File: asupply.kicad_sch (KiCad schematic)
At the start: 73 parts

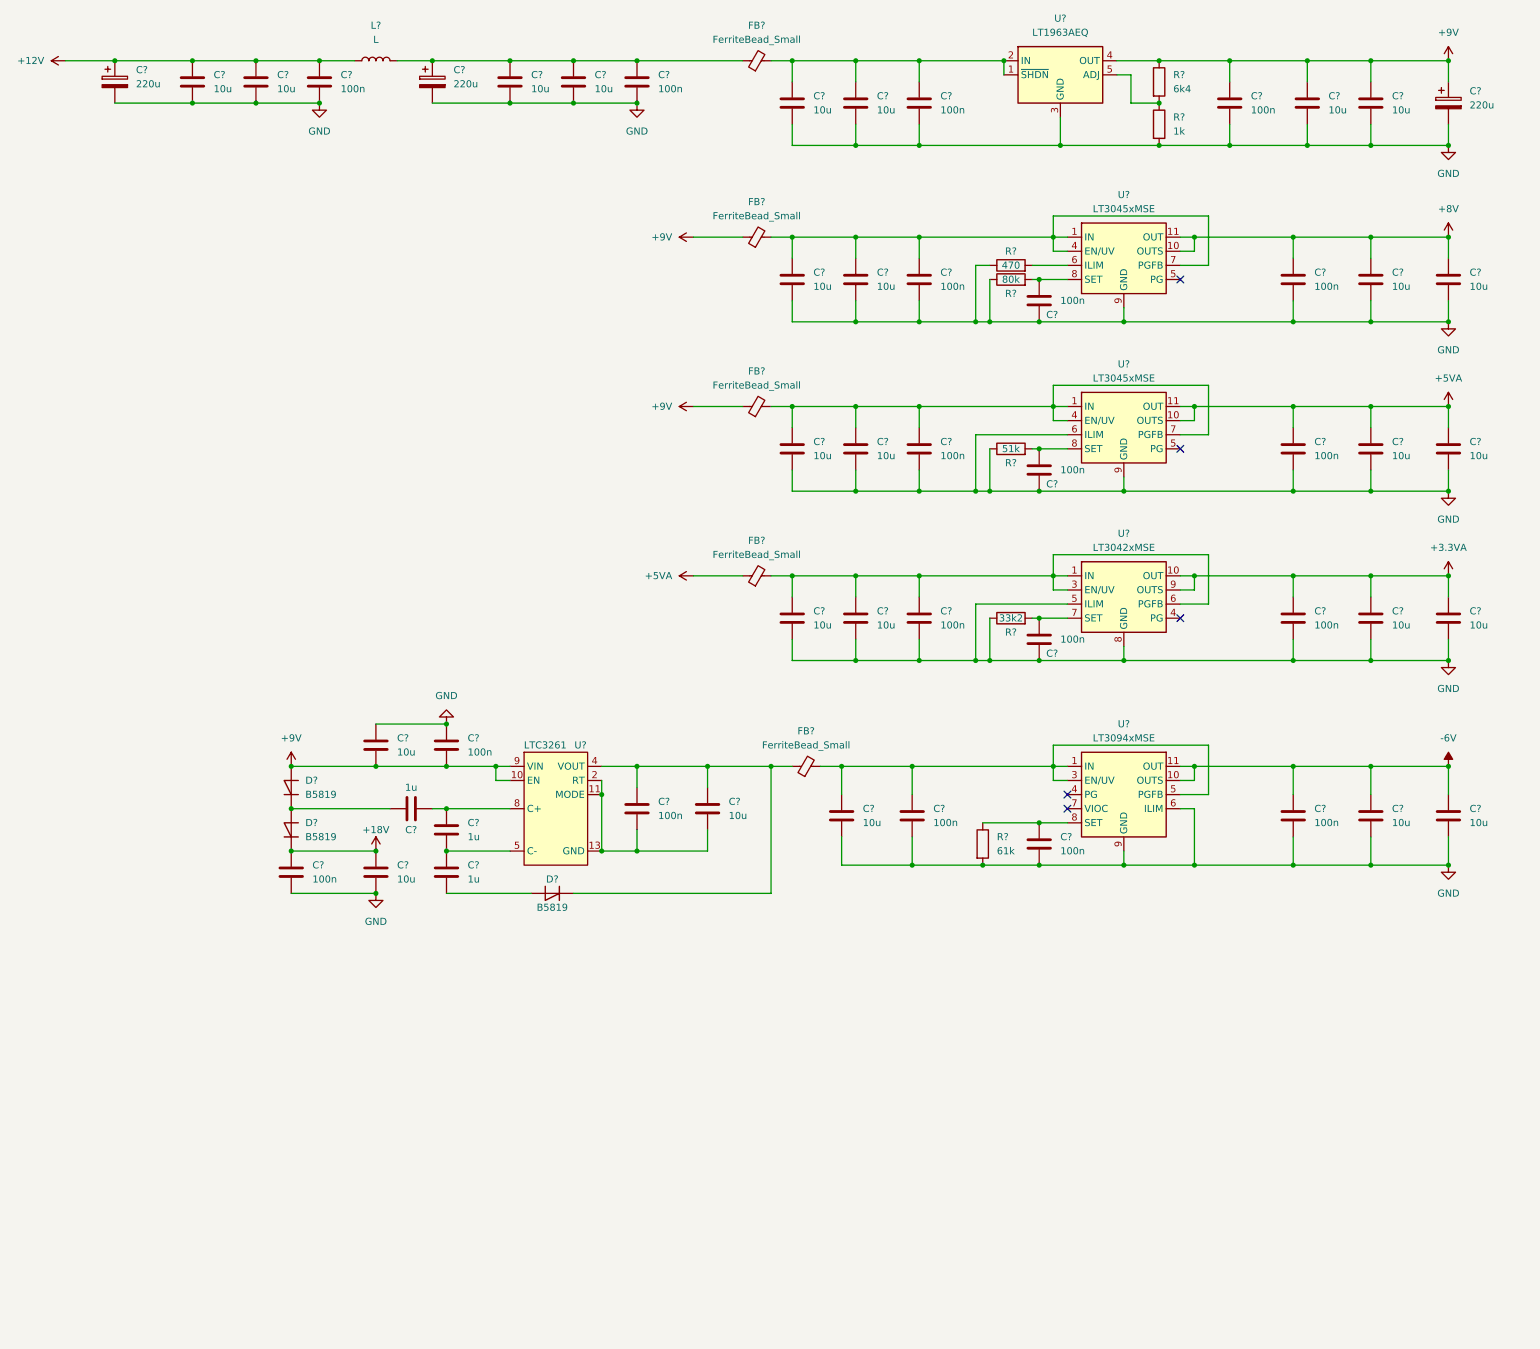
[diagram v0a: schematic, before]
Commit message: analog supply complete
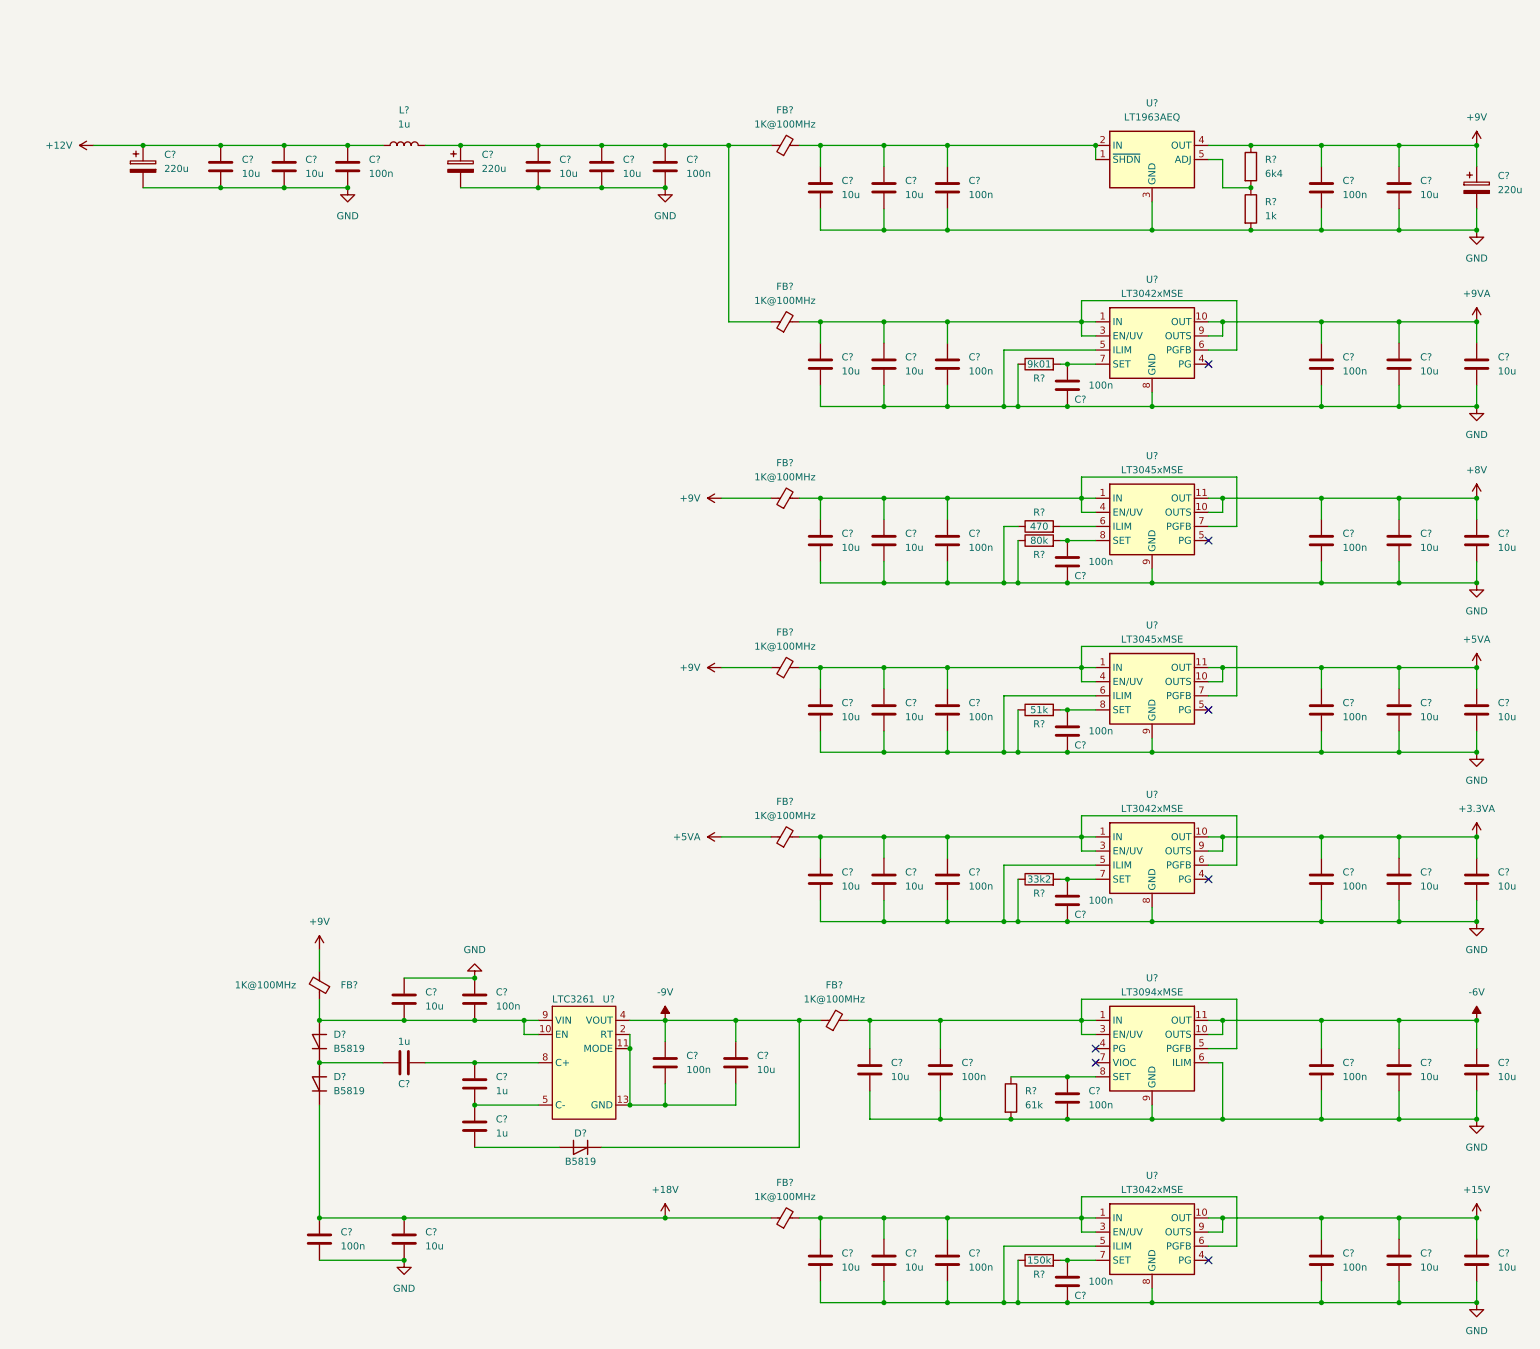
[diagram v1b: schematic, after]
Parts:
- removed C?: 10u, symbol Device:C
- removed FB? (x4): FerriteBead_Small, symbol Device:FerriteBead_Small
- added C? (x6): 100n, symbol Device:C
- added C? (x8): 10u, symbol Device:C
- added FB? (x7): 1K@100MHz, symbol Device:FerriteBead_Small
- added R?: 9k01, symbol Device:R
- added R?: 150k, symbol Device:R
- added U? (x2): LT3042xMSE, Package_SO:MSOP-10-1EP_3x3mm_P0.5mm_EP1.68x1.88mm, symbol Regulator_Linear:LT3042xMSE
- FB?: value FerriteBead_Small -> 1K@100MHz
- L?: value L -> 1u
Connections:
- net +1V8: now also FB?.1
- net +5VA: now also FB?.1
- net +9V: now also FB?.1, FB?.1, FB?.2; no longer C?.2, C?.2, D?.2 (A), U?.10 (EN), U?.9 (VIN)
- net GND: now also C?.2, C?.2, C?.2, C?.2, C?.2, C?.2, C?.2, C?.2, C?.2, C?.2, C?.2, C?.2, C?.2, C?.2, R?.1, R?.1, U?.11 (GND), U?.11 (GND), U?.5 (ILIM), U?.5 (ILIM), U?.8 (GND), U?.8 (GND)
- net -9V: now reaches C?.1, C?.1, D?.1 (K), U?.4 (VOUT)
- net -9V: now also FB?.1
- net at C?.1, C?.1, C?.1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: now also FB?.1
- net at C?.1, C?.1, C?.1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: now also FB?.2 (x2)
- net at C?.1, C?.1, C?.1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: now also FB?.2
- net at C?.1, C?.1, U?.1 (IN)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: now also FB?.2
- new net: C?.1, R?.2, U?.7 (SET) (x2)
- new net: C?.1, C?.1, C?.1, FB?.2, U?.1 (IN), U?.2 (IN), U?.3 (EN/UV), U?.6 (PGFB) (x2)
- new net: C?.2, C?.2, D?.2 (A), FB?.1, U?.10 (EN), U?.9 (VIN)
- new net +15V: C?.1, C?.1, C?.1, U?.10 (OUT), U?.9 (OUTS)
- new net +9VA: C?.1, C?.1, C?.1, U?.10 (OUT), U?.9 (OUTS)
- no-connect marks 5 -> 7
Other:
- moved on the sheet: C?, D?, FB?, L?, R?, U?
